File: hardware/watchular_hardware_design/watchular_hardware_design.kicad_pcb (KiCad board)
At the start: 4 copper layers, 55.5 x 22.9 mm, 90 parts, among them J1 USB4105-GF-A, J2 665102131822, J3 TSW-116-07-H-S, J4 TSW-116-07-H-S, Q1 BSS123, Q2 BSS123, Q3 BSS123, Q4 BSS123, T1 DMG1013UW-7, U1 MCP73832T-2DCI/OT, U2 ESP32-C3FH4, U3 MIC5524-3.3YMT-TZ, U4 W25Q16JVSSIQ, U5 TL3305AF260QG, U6 TL3305AF260QG, Y1 40MHz

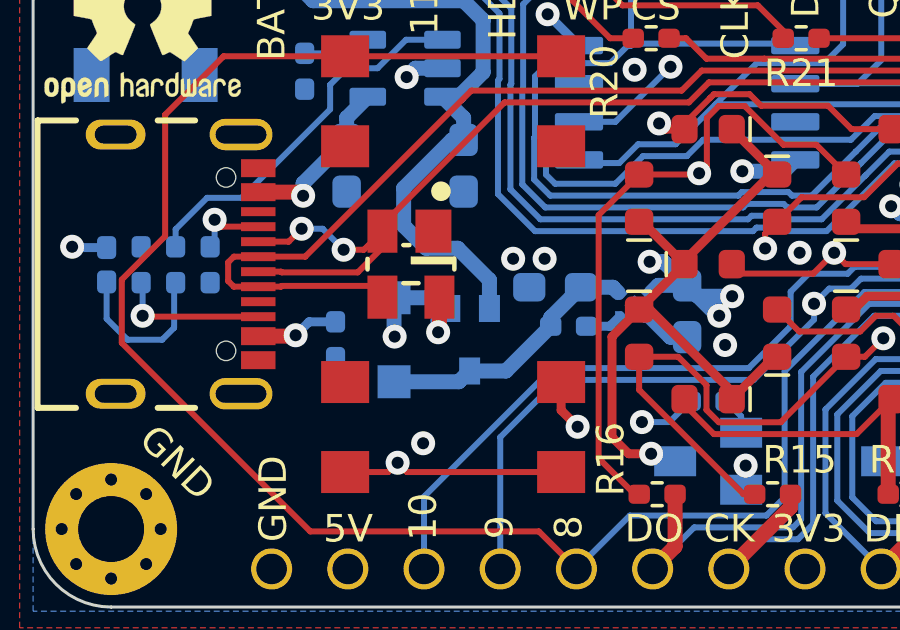
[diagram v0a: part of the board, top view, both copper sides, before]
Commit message: Started the BOM.
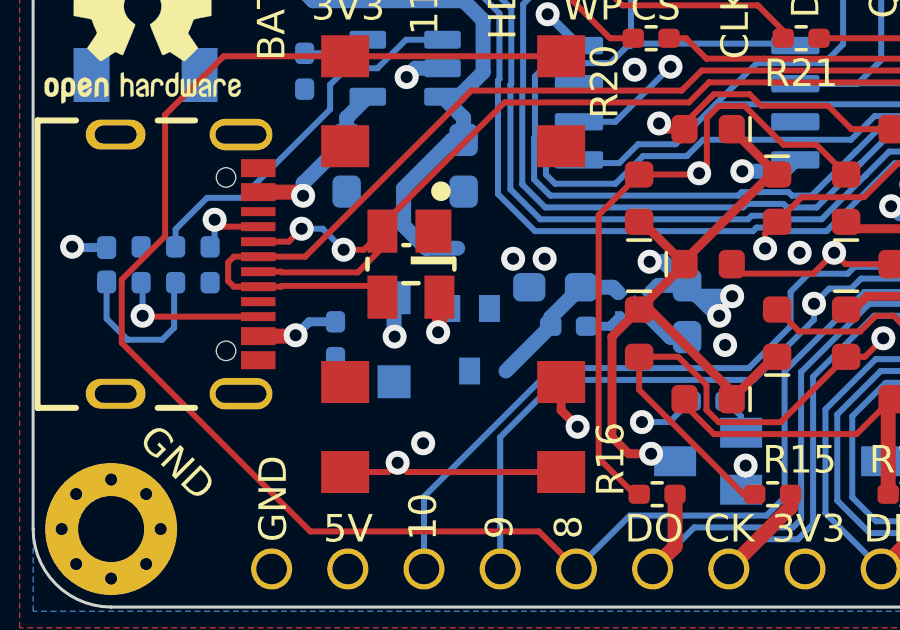
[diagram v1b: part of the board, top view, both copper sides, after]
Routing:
- net VCC: track 9.02 -> 5.14 mm
- net +5V: track 15.3 -> 12.4 mm
- net +BATT: track 25.2 -> 22.8 mm
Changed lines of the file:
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@@
   (segment (start 100.45 117.2875) (end 99 118.7375) (width 0.5) (layer "B.Cu") (net 21))
   (segment (start 102.03 123.824502) (end 102.05 123.844502) (width 0.5) (layer "B.Cu") (net 21))
-  (segment (start 103.5 123.2982) (end 103.8896 122.9086) (width 0.5) (layer "B.Cu") (net 21))
-  (segment (start 102.03 122.55) (end 103.531 122.55) (width 0.5) (layer "B.Cu") (net 21))
   (segment (start 91.3275 120.8775) (end 91.3 120.85) (width 0.3) (layer "B.Cu") (net 21))
-  (segment (start 103.531 122.55) (end 103.8896 122.9086) (width 0.5) (layer "B.Cu") (net 21))
   (segment (start 100.08 123.3525) (end 99.1975 123.3525) (width 0.3) (layer "B.Cu") (net 21))
   (segment (start 99 118.7375) (end 99 119.15) (width 0.5) (layer "B.Cu") (net 21))
   (segment (start 92.45 120.8775) (end 91.3275 120.8775) (width 0.3) (layer "B.Cu") (net 21))
-  (segment (start 103.5 123.7) (end 103.5 123.2982) (width 0.5) (layer "B.Cu") (net 21))
   (segment (start 100.45 116.555) (end 101.155 115.85) (width 0.5) (layer "B.Cu") (net 21))
   (segment (start 99.1975 123.3525) (end 98.75 123.8) (width 0.3) (layer "B.Cu") (net 21))
@@
   (segment (start 94.25 111.25) (end 97.93 111.25) (width 0.5) (layer "B.Cu") (net 45))
   (segment (start 99.33 112.65) (end 97.95 111.27) (width 0.5) (layer "B.Cu") (net 45))
-  (segment (start 105.2104 121.9586) (end 104.1518 120.9) (width 0.5) (layer "B.Cu") (net 45))
   (segment (start 102.35 120.15) (end 102.35 118.9) (width 0.5) (layer "B.Cu") (net 45))
   (segment (start 104.35 116.555) (end 103.645 115.85) (width 0.5) (layer "B.Cu") (net 45))
   (segment (start 102.35 118.9) (end 103.9625 117.2875) (width 0.5) (layer "B.Cu") (net 45))
-  (segment (start 105.2104 122.9086) (end 105.2104 121.9586) (width 0.5) (layer "B.Cu") (net 45))
   (segment (start 103.9625 117.2875) (end 104.35 117.2875) (width 0.5) (layer "B.Cu") (net 45))
   (segment (start 105 115.031604) (end 105 113.3) (width 0.5) (layer "B.Cu") (net 45))
@@
   (segment (start 125.7875 124.16) (end 127.35 122.5975) (width 0.2) (layer "F.Cu") (net 54))
   (segment (start 109.325 122.2) (end 109.503131 122.378131) (width 0.5) (layer "B.Cu") (net 55))
-  (segment (start 104.55 124.9914) (end 105.7611 124.9914) (width 0.5) (layer "B.Cu") (net 55))
-  (segment (start 104.1914 125.35) (end 104.55 124.9914) (width 0.5) (layer "B.Cu") (net 55))
   (segment (start 105.7611 124.9914) (end 107.2525 123.5) (width 0.5) (layer "B.Cu") (net 55))
   (segment (start 107.2525 123.5) (end 107.2525 123.21) (width 0.5) (layer "B.Cu") (net 55))
   (segment (start 107.2525 123.21) (end 108.2625 122.2) (width 0.5) (layer "B.Cu") (net 55))
   (segment (start 108.2625 122.2) (end 109.325 122.2) (width 0.5) (layer "B.Cu") (net 55))
-  (segment (start 102.03 125.35) (end 104.1914 125.35) (width 0.5) (layer "B.Cu") (net 55))
   (segment (start 108.4475 123.5) (end 109.225 123.5) (width 0.3) (layer "B.Cu") (net 56))
   (segment (start 109.225 123.5) (end 109.573842 123.151158) (width 0.3) (layer "B.Cu") (net 56))
